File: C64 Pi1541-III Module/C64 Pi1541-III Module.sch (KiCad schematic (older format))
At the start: 21 parts, among them J1 DC IN, J2 C64_IEC, J3 C64_IEC, J8 Module_Panel, M1 Mounting, M2 Mounting, M3 Mounting, M4 Mounting, U1 7406

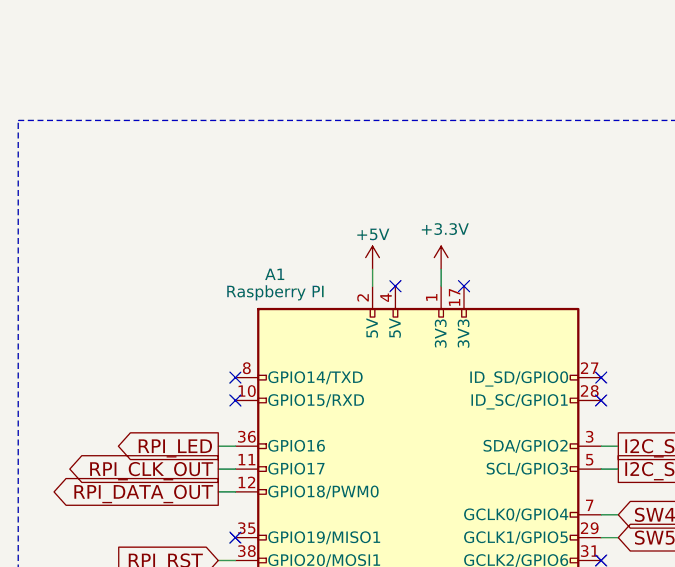
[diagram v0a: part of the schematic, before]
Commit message: Exported files
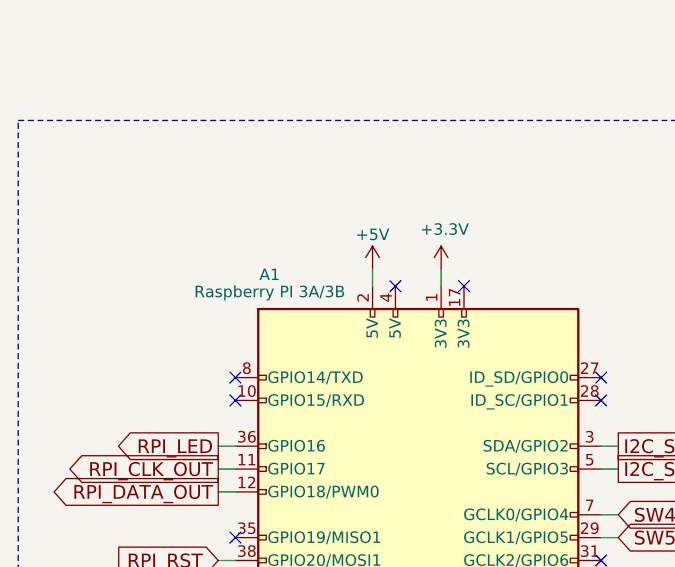
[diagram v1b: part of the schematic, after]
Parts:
- A1: value Raspberry PI -> Raspberry PI 3A/3B
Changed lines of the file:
@@
 U 1 1 640CCE33
 P 2725 3400
-F 0 "A1" H 2100 4750 50  0000 C CNN
-F 1 "Raspberry PI" H 2100 4675 50  0000 C CNN
+F 0 "A1" H 2075 4750 50  0000 C CNN
+F 1 "Raspberry PI 3A/3B" H 2075 4675 50  0000 C CNN
 F 2 "RPI:Raspberry_Pi_3B_Socketed_THT_FaceDown_MountingHoles" H 2725 3400 50  0001 C CNN
 F 3 "https://www.raspberrypi.org/documentation/hardware/raspberrypi/schematics/rpi_SCH_3bplus_1p0_reduced.pdf" H 2725 3400 50  0001 C CNN
